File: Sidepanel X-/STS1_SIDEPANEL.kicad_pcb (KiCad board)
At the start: 2 copper layers, 82.8 x 100 mm, 30 parts, among them IC1 TMP112AQDRLRQ1, J1 Conn_02x04_Odd_Even, J2 Conn_02x02_Odd_Even, U1 GUVA-C32SM

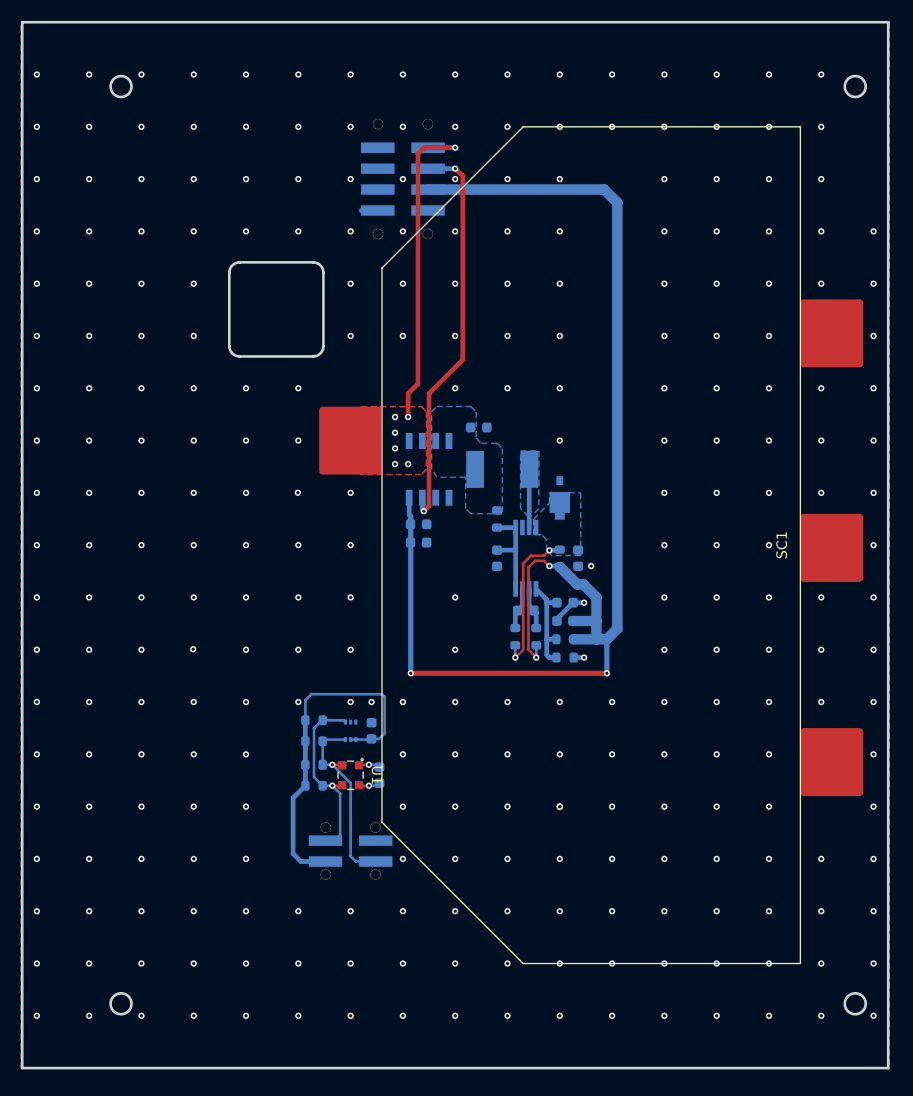
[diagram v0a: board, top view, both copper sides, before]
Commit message: Review Ready for V2.0
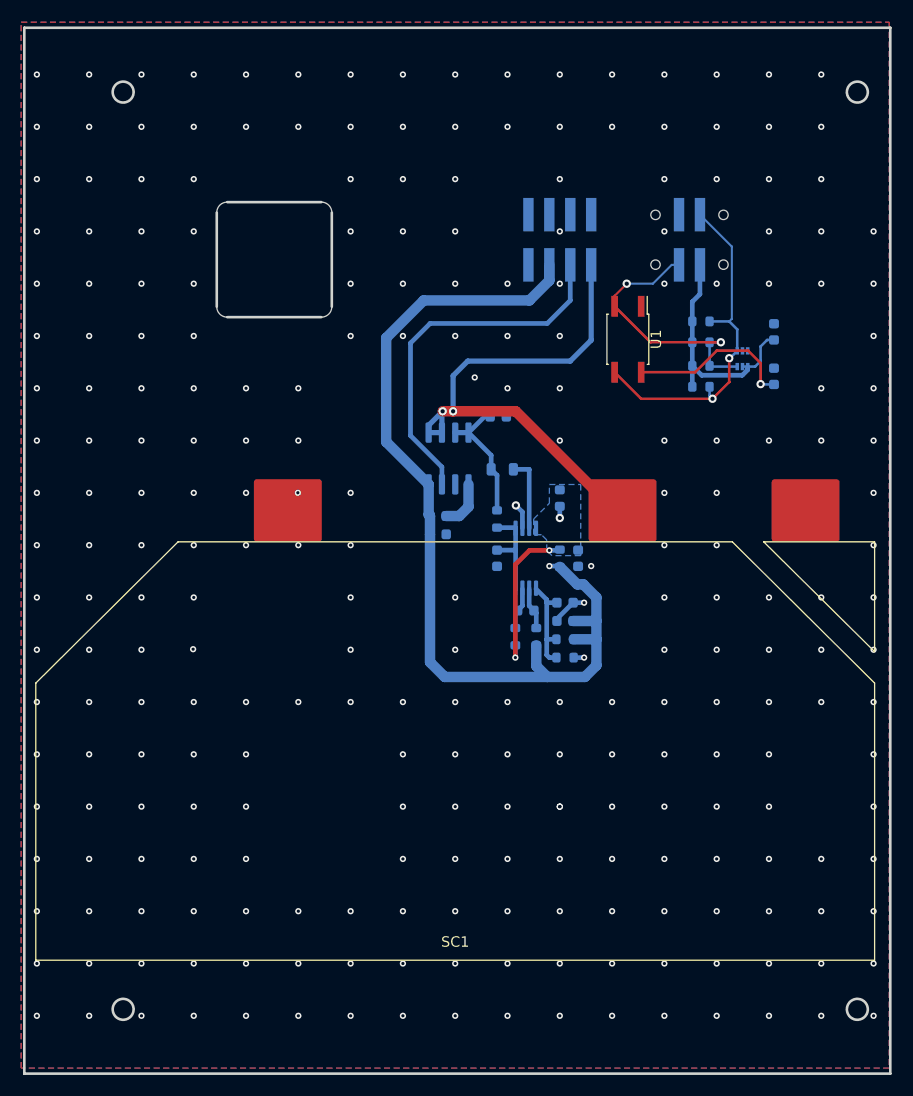
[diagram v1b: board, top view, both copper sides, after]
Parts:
- CUR1: footprint SamacSys:SOIC127P600X175-8N -> Package_SO:SOIC-8_3.9x4.9mm_P1.27mm
- DOUT1: footprint SamacSys:STMITE -> Diode_SMD:D_0603_1608Metric
- IC1: footprint SamacSys:SOTFL50P160X60-6N -> Package_TO_SOT_SMD:SOT-563
- J1: footprint SamacSys:M808280842 -> STS_Connector:M808280842
- J2: footprint USER_Passiv:M80-8280442 -> STS_Connector:M808280442
- L_IN1: footprint SamacSys:INDPM5650X530N -> Inductor_SMD:L_0805_2012Metric
- MPPT1: footprint SamacSys:SOP65P640X120-8N -> Package_SO:TSSOP-8_4.4x3mm_P0.65mm
- U1: footprint USER_Optic:OLGA 2mm x 2,3mm -> Package_SO:SO-4_4.4x3.6mm_P2.54mm
- moved J2 66.8 mm to (147.4, 60.3), turned to 180 degrees
- moved C2 54.2 mm to (155.5, 69.1)
- moved C1 53.7 mm to (155.5, 73.4)
- moved RIC1 53.1 mm to (148.5, 68.1)
- moved RIC2 53.1 mm to (148.5, 70.1)
- moved RU1 53.1 mm to (148.5, 74.4)
- moved RU2 53.1 mm to (148.5, 72.4)
- moved IC1 51.7 mm to (152.5, 71.7)
- moved U1 49.4 mm to (141.5, 69.8)
- moved SC1 23.6 mm to (125.0, 109.2), turned to 0 degrees
- moved J1 16.1 mm to (135.0, 60.3), turned to 180 degrees
- moved C_IN1 2.13 mm to (129.1, 77.2)
- moved CUR1 2.13 mm to (124.4, 81.2)
- moved C_CUR11 2.02 mm to (123.4, 86.7)
- moved C_CUR21 2.02 mm to (123.4, 88.5)
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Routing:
- net /MPPT1: track 127.5 -> 89.2 mm, vias 4 -> 1
- net /SC1_V+: track 32.0 -> 52.3 mm, vias 7 -> 2
- net /SCL: track 17.8 -> 33.9 mm, vias 1 -> 2
- net /Sensors/VBAT: track 2.06 -> 16.1 mm
- net /SolarMPPT/CUR1_OUT: track 0.00 -> 12.5 mm
- net /+3V3: track 33.2 -> 23.2 mm
- net /SDA: track 18.5 -> 26.0 mm, vias 1 -> 2
- net GND: track 6.50 -> 12.6 mm, vias 282 -> 262
- net /SC1_I+: track 38.6 -> 35.1 mm, vias 2 -> 0
- net /SC2_V+: track 1.60 -> 0.00 mm
- net /SolarMPPT/MPPT1_IN: track 6.57 -> 7.17 mm
- removed copper zone on B.Cu, net /SC1_V+
- removed copper zone on F.Cu, net /SC1_V+
- removed copper zone on B.Cu, net /SolarMPPT/CUR1_OUT
- removed copper zone on B.Cu, net /SolarMPPT/MPPT1_IN
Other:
- outline, holes or cut-outs redrawn
